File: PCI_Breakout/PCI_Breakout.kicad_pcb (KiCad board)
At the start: 2 copper layers, 74 x 36 mm, 2 parts, among them J1 凹

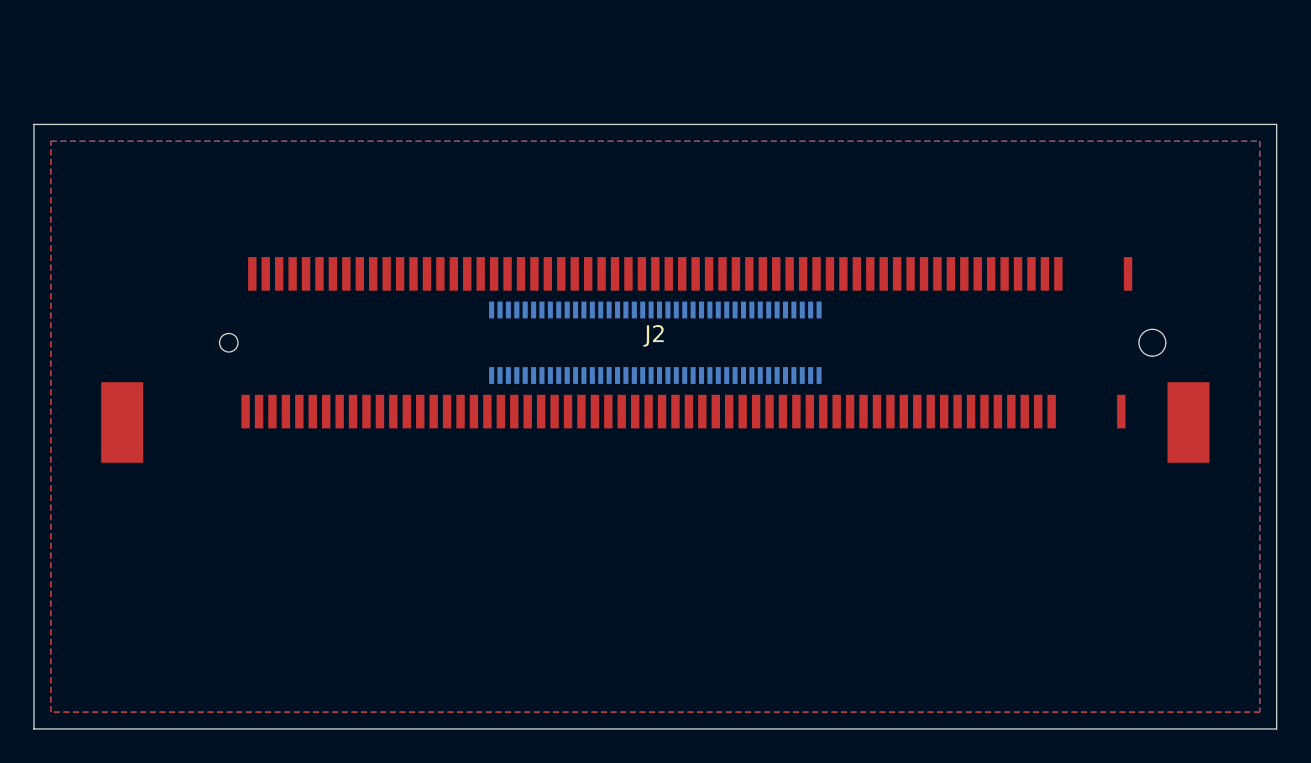
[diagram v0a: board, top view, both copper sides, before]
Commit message: pci
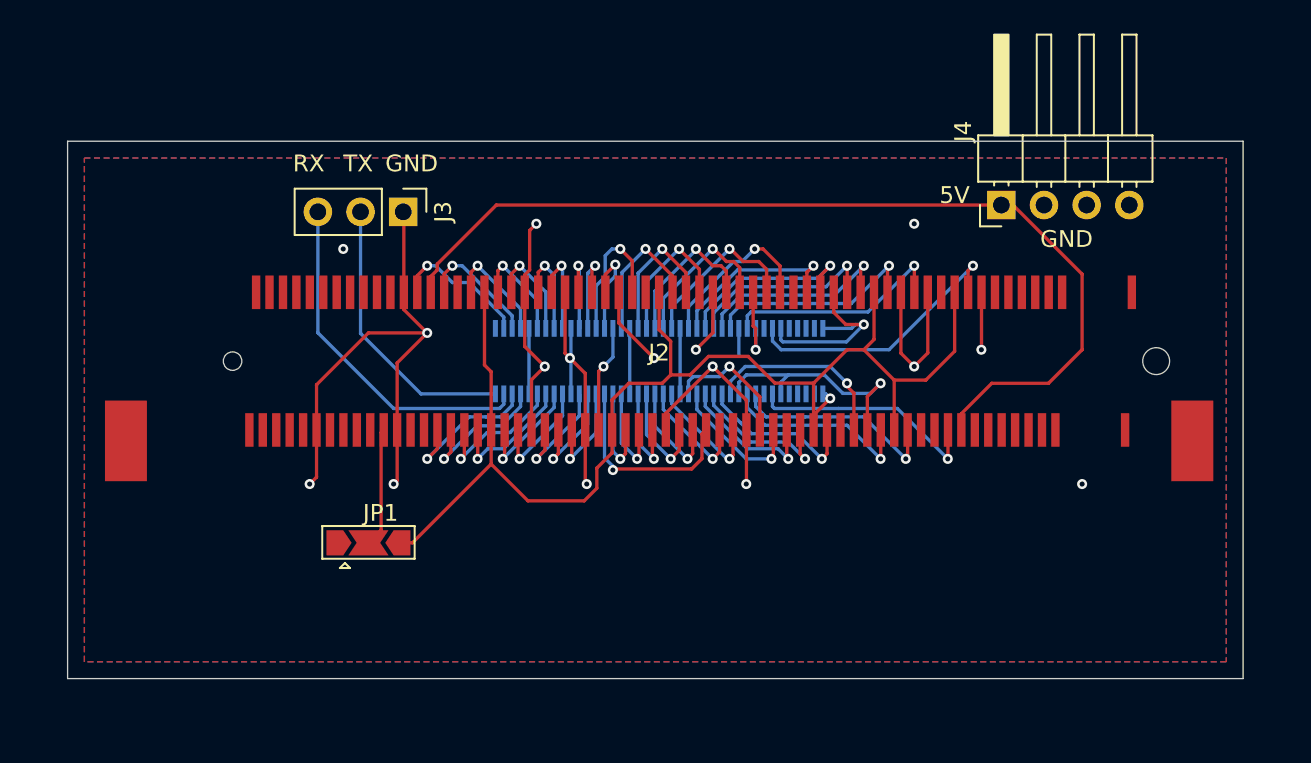
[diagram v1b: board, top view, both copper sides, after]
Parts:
- added J3: Conn_01x03_Pin, Connector_PinHeader_2.54mm:PinHeader_1x03_P2.54mm_Vertical, F.Cu at (115.6, 97.8)
- added J4: Conn_01x04_Pin, Connector_PinHeader_2.54mm:PinHeader_1x04_P2.54mm_Horizontal, F.Cu at (151.2, 97.4)
- added JP1: Jumper_3_Open, Jumper:SolderJumper-3_P2.0mm_Open_TrianglePad1.0x1.5mm, F.Cu at (113.5, 117.5)
- moved J1 1.12 mm to (130.8, 106.7)
- moved J2 1.12 mm to (130.8, 106.7)
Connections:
- J1 pad 2: +3.3V_BRIDGE -> +3.3V
- J1 pad 34: unconnected-(J1-Pin_34-Pad34) -> SB_PCI_IDSEL
- J2 pad 104: unconnected-(J2-M66EN-Pad104) -> Net-(J2-M66EN)
- J2 pad 48: unconnected-(J2-IDSEL-Pad48) -> SB_PCI_IDSEL
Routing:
- net GND: track 0.00 -> 139.5 mm, vias 0 -> 19
- net +3.3V: track 0.00 -> 76.2 mm, vias 0 -> 1
- net +5V: track 0.00 -> 57.6 mm
- net SB_SIO0_RXD: track 0.00 -> 20.9 mm
- net SB_SIO0_TXD: track 0.00 -> 16.8 mm
- net SB_PCI_INTB: track 0.00 -> 16.7 mm, vias 0 -> 1
- net SB_PCI_INTA: track 0.00 -> 14.2 mm, vias 0 -> 1
- net SB_PCI0_CLK: track 0.00 -> 13.5 mm, vias 0 -> 1
- net SB_PCI_REQ0: track 0.00 -> 13.1 mm, vias 0 -> 1
- net SB_PCI_RST: track 0.00 -> 12.7 mm, vias 0 -> 1
- net SB_PCI_PAR: track 0.00 -> 12.2 mm, vias 0 -> 1
- net SB_PCI_AD31: track 0.00 -> 12.1 mm, vias 0 -> 1
- net SB_PCI_GNT0: track 0.00 -> 11.7 mm, vias 0 -> 1
- net SB_PCI_AD29: track 0.00 -> 11.6 mm, vias 0 -> 1
- net SB_PCI_PME: track 0.00 -> 11.4 mm, vias 0 -> 1
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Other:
- board size 74 x 36 mm -> 70 x 32 mm
- board text added: "5V"
- board text added: "GND"
- board text added: "RX"
- board text added: "TX"
